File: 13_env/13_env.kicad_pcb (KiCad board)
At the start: 2 copper layers, 30 x 100 mm, 53 parts, among them J1 gate in 1, J5 env out 1, J6 End of Cycle Out, Q1 BC848, Q2 BC858, Q3 BC848, Q4 BC858, SW1 Manual Gate, SW2 Normal/Inverted, SW4 Gate/Loop, U1 TL074, U2 TL072

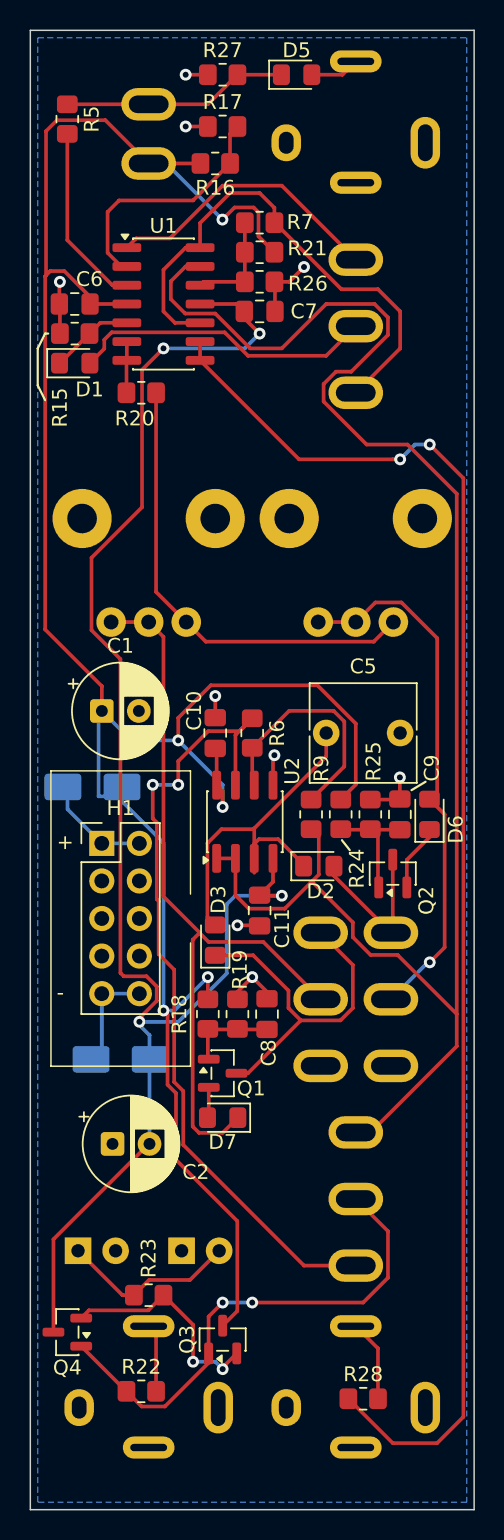
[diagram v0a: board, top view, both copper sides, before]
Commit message: updated 13 pcb
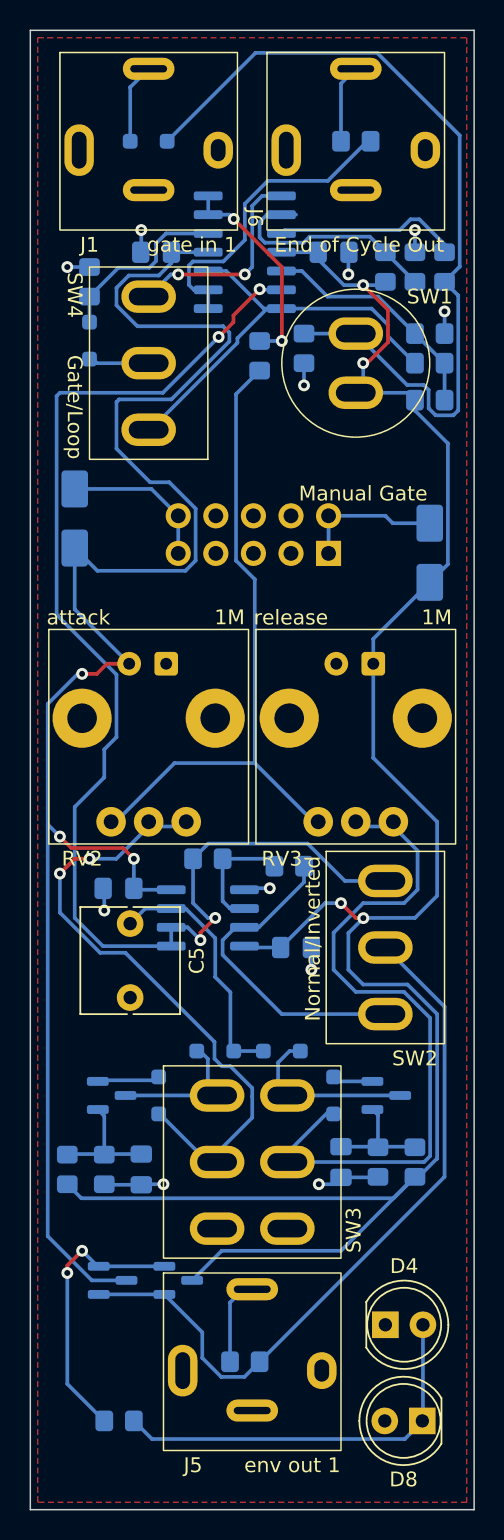
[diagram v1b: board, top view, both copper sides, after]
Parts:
- C1, C2, H1, Q1, Q2, Q3, Q4, U1, U2: moved to B.Cu
- C10, C11, C6, C7, C8, C9: footprint Capacitor_SMD:C_0805_2012Metric_Pad1.18x1.45mm_HandSolder -> cynthia:C SMD 0805; moved to B.Cu
- D1, D2, D3, D5, D6, D7: footprint Diode_SMD:D_0805_2012Metric_Pad1.15x1.40mm_HandSolder -> Diode_SMD:D_SOD-323_HandSoldering; moved to B.Cu
- D4, D8, J1, J5, J6, RV2, RV3, SW1, SW2, SW3, SW4: moved to F.Cu
- R15, R16, R17, R18, R19, R20, R21, R22, R23, R24, R25, R26, R27, R28, R5, R6, R7, R9: footprint Resistor_SMD:R_0805_2012Metric_Pad1.20x1.40mm_HandSolder -> cynthia:R SMD 0805; moved to B.Cu
- moved R28 85.0 mm to (17.0, 12.0), turned to 180 degrees
- moved J6 85.0 mm to (17.0, 12.0), turned to 0 degrees
- moved D11 36.7 mm to (-2.00, 37.5), turned to -90 degrees
- moved C2 32.7 mm to (4.18, 47.3), turned to 180 degrees
- moved R24 30.3 mm to (-2.50, 81.5), turned to -90 degrees
- moved R25 30.0 mm to (0.00, 81.5), turned to 90 degrees
- moved C9 29.7 mm to (2.50, 81.5), turned to -90 degrees
- moved D12 27.8 mm to (22.0, 39.8), turned to 90 degrees
- moved R5 27.4 mm to (23.0, 20.5), turned to 90 degrees
- moved D6 26.4 mm to (3.67, 76.5), turned to -90 degrees
- moved D8 26.0 mm to (21.5, 98.5), turned to 180 degrees
- moved H1 24.9 mm to (15.2, 39.9), turned to 90 degrees
- moved Q2 24.2 mm to (0.50, 76.5), turned to 0 degrees
- moved SW1 20.9 mm to (17.0, 27.0), turned to 0 degrees
- moved RV2 19.4 mm to (3.00, 51.0), turned to 0 degrees
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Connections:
- R20 pad 1: Net-(U1B--) -> Net-(U1D--)
- R21 pad 1: Net-(U1D-+) -> Net-(U1B-+)
- R26 pad 2: Net-(U1D-+) -> Net-(U1B-+)
- R7 pad 1: Net-(U1D-+) -> Net-(U1B-+)
- U1 pad 12: Net-(U1D-+) -> Net-(D1-K)
- U1 pad 13: Net-(SW2-A) -> Net-(U1D--)
- U1 pad 14: Net-(SW4-A) -> Net-(U1D--)
- U1 pad 5: Net-(D1-K) -> Net-(U1B-+)
- U1 pad 6: Net-(U1B--) -> Net-(SW2-A)
- U1 pad 7: Net-(U1B--) -> Net-(SW4-A)
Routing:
- net Net-(U1C--): track 96.4 -> 21.2 mm, vias 2 -> 0
- net Net-(D5-K): track 15.3 -> 57.5 mm
- net Net-(SW2-C): track 55.1 -> 21.9 mm, vias 2 -> 0
- net Net-(SW2-A): track 115.4 -> 88.8 mm, vias 0 -> 4
- net +12V: track 161.7 -> 140.4 mm, vias 5 -> 4
- net Net-(D1-A): track 20.7 -> 4.21 mm
- net Net-(U1B-+): track 0.00 -> 16.0 mm
- net Net-(Q3-B): track 34.1 -> 49.5 mm, vias 2 -> 0
- net Net-(D4-A): track 12.0 -> 27.1 mm
- net Net-(U1D--): track 0.00 -> 14.2 mm, vias 0 -> 2
- net Net-(R20-Pad2): track 31.4 -> 45.6 mm
- net -12V: track 107.1 -> 119.8 mm, vias 4 -> 3
- net Net-(D3-K): track 24.0 -> 12.3 mm
- net Net-(D2-K): track 26.0 -> 17.0 mm
- net Net-(U2B--): track 16.9 -> 8.05 mm
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- added copper zone on F.Cu, net GND
- removed copper zone on B.Cu, net GND
